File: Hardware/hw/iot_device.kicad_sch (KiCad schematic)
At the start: 19 parts, among them J4 Screw_Terminal_01x02, J6 Screw_Terminal_01x02, U1 ESP32-C6-WROOM-1, U2 RV-3028-C7, U5 TPS63001

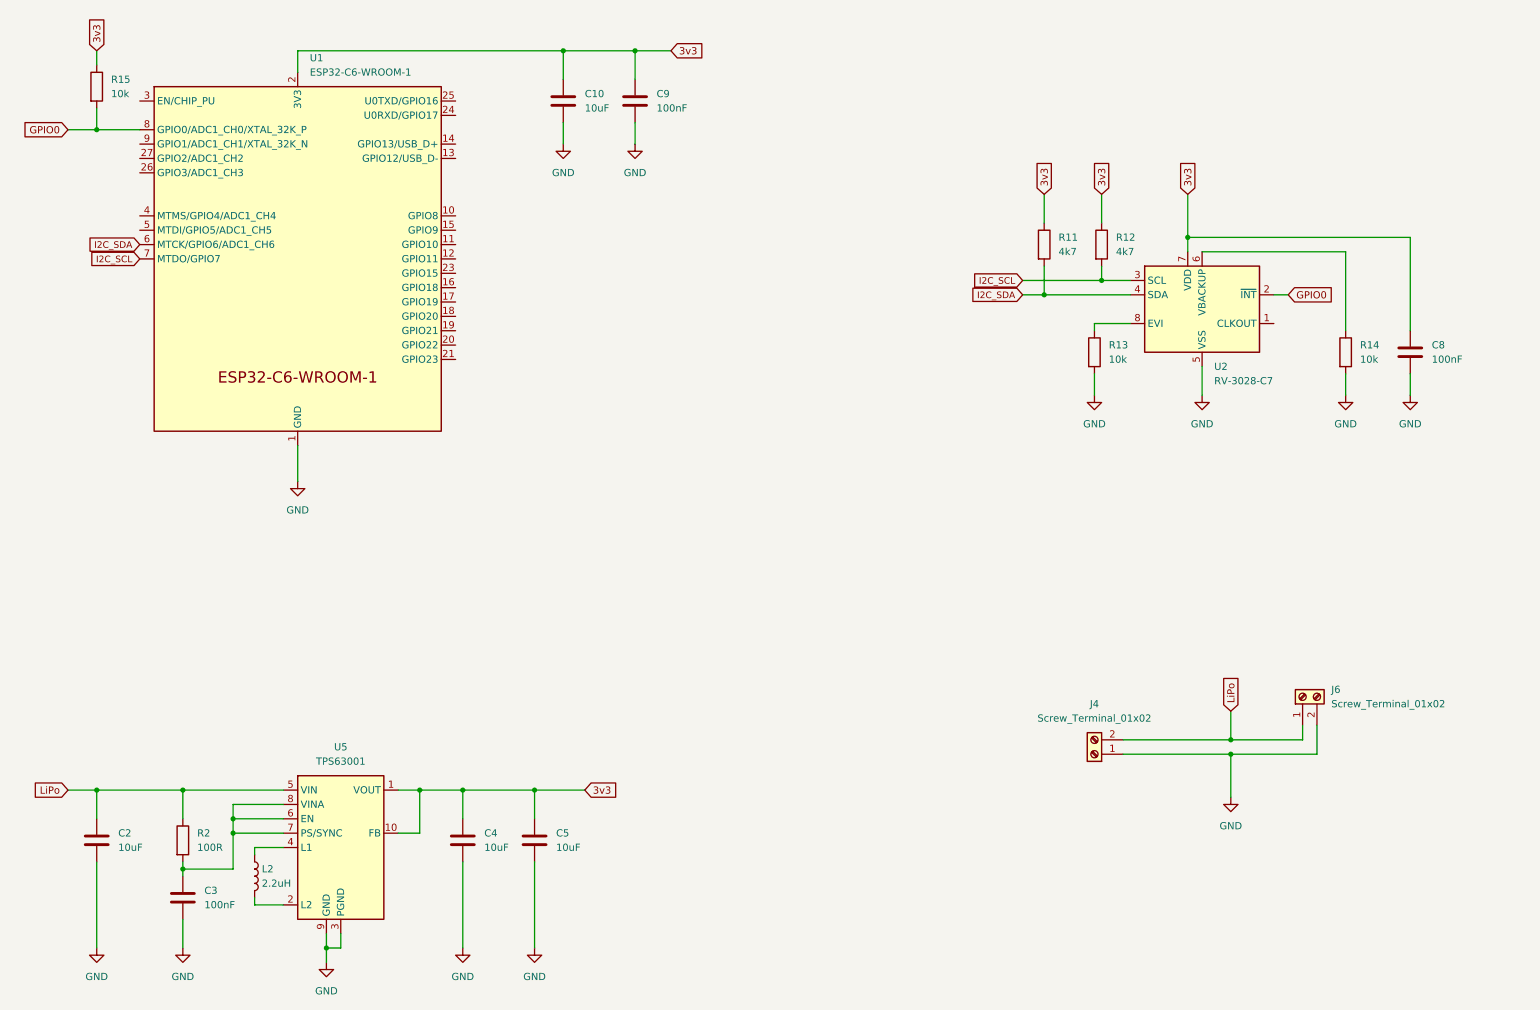
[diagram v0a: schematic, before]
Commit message: IoT update
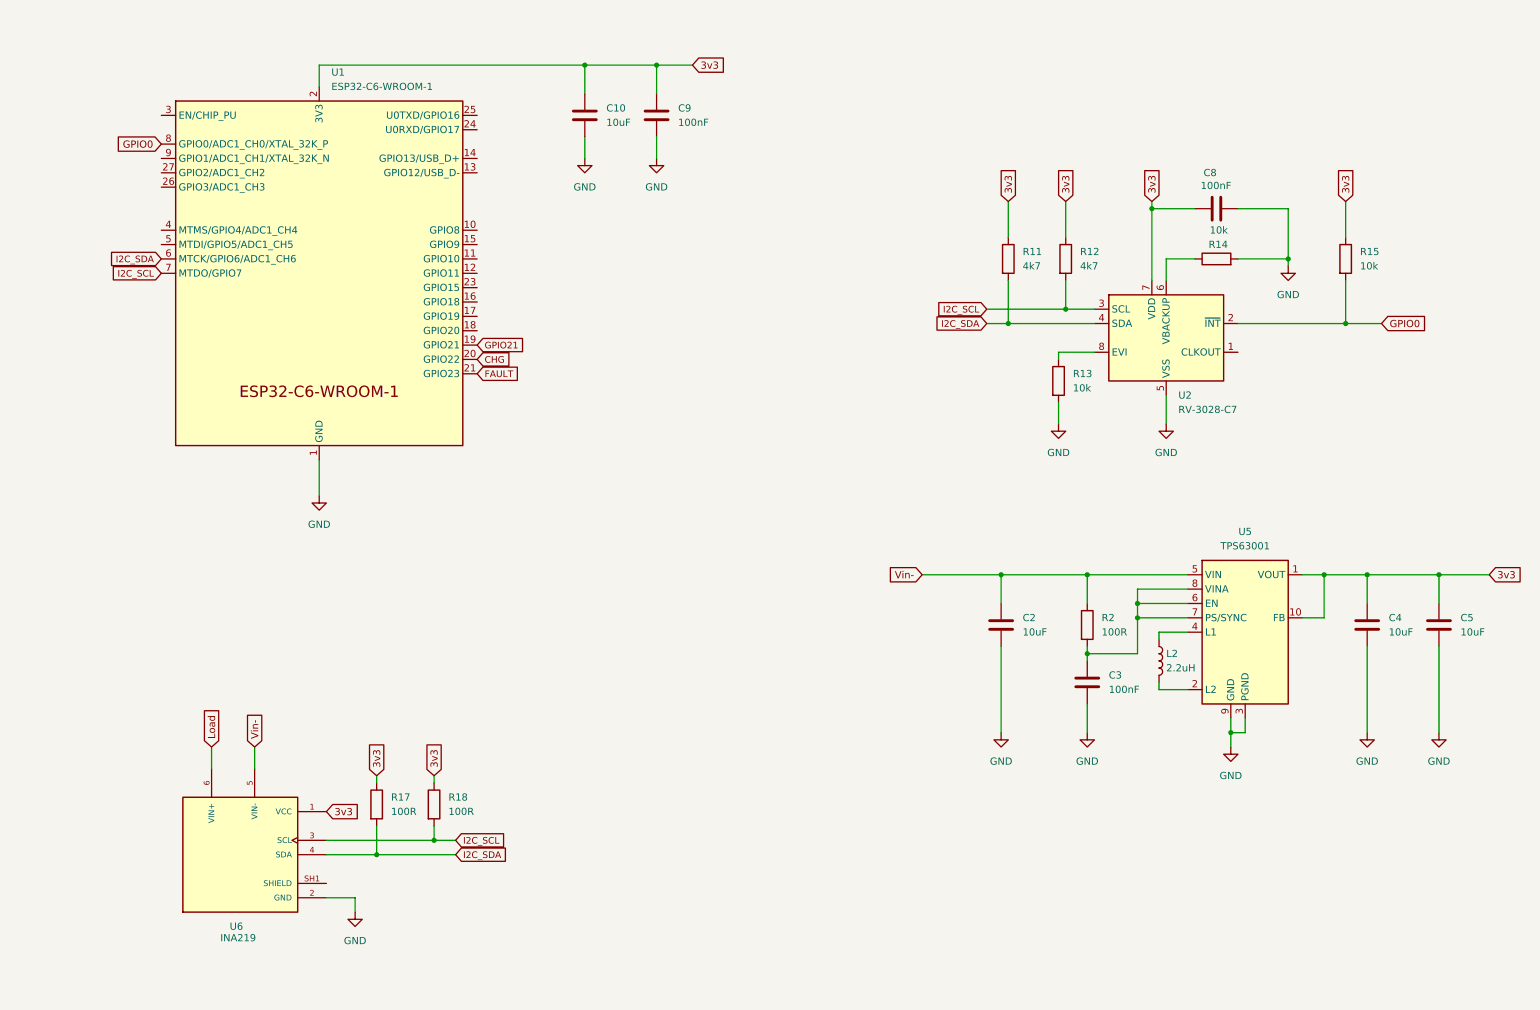
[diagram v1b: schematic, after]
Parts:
- removed J4, J6: Screw_Terminal_01x02, TerminalBlock_Phoenix:TerminalBlock_Phoenix_MPT-0,5-2-2.54_1x02_P2.54mm_Horizontal, symbol Connector:Screw_Terminal_01x02
- added R17, R18: 100R, Resistor_SMD:R_0805_2012Metric, symbol Device:R
- added U6: INA219, INA219_Module:MODULE_INA219, symbol INA219:INA219
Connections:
- net 3v3: now also C8.1, R17.1, R18.1, U6.1 (VCC); no longer C8.2
- net GND: now also C8.2, U6.2 (GND); no longer C8.1
- net I2C_SCL: now also R18.2, U6.3 (SCL)
- net I2C_SDA: now also R17.2, U6.4 (SDA)
- net GPIO21: now reaches U1.19 (GPIO21)
- net CHG: now reaches U1.20 (GPIO22)
- net FAULT: now reaches U1.21 (GPIO23)
- net LiPo renamed Vin-
- net Vin-: now also U6.5 (VIN-)
- new net Load: U6.6 (VIN+)
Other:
- moved on the sheet: C10, C2, C3, C4, C5, C8, C9, L2, R11, R12, R13, R14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
